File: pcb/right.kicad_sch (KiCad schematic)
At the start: 0 parts

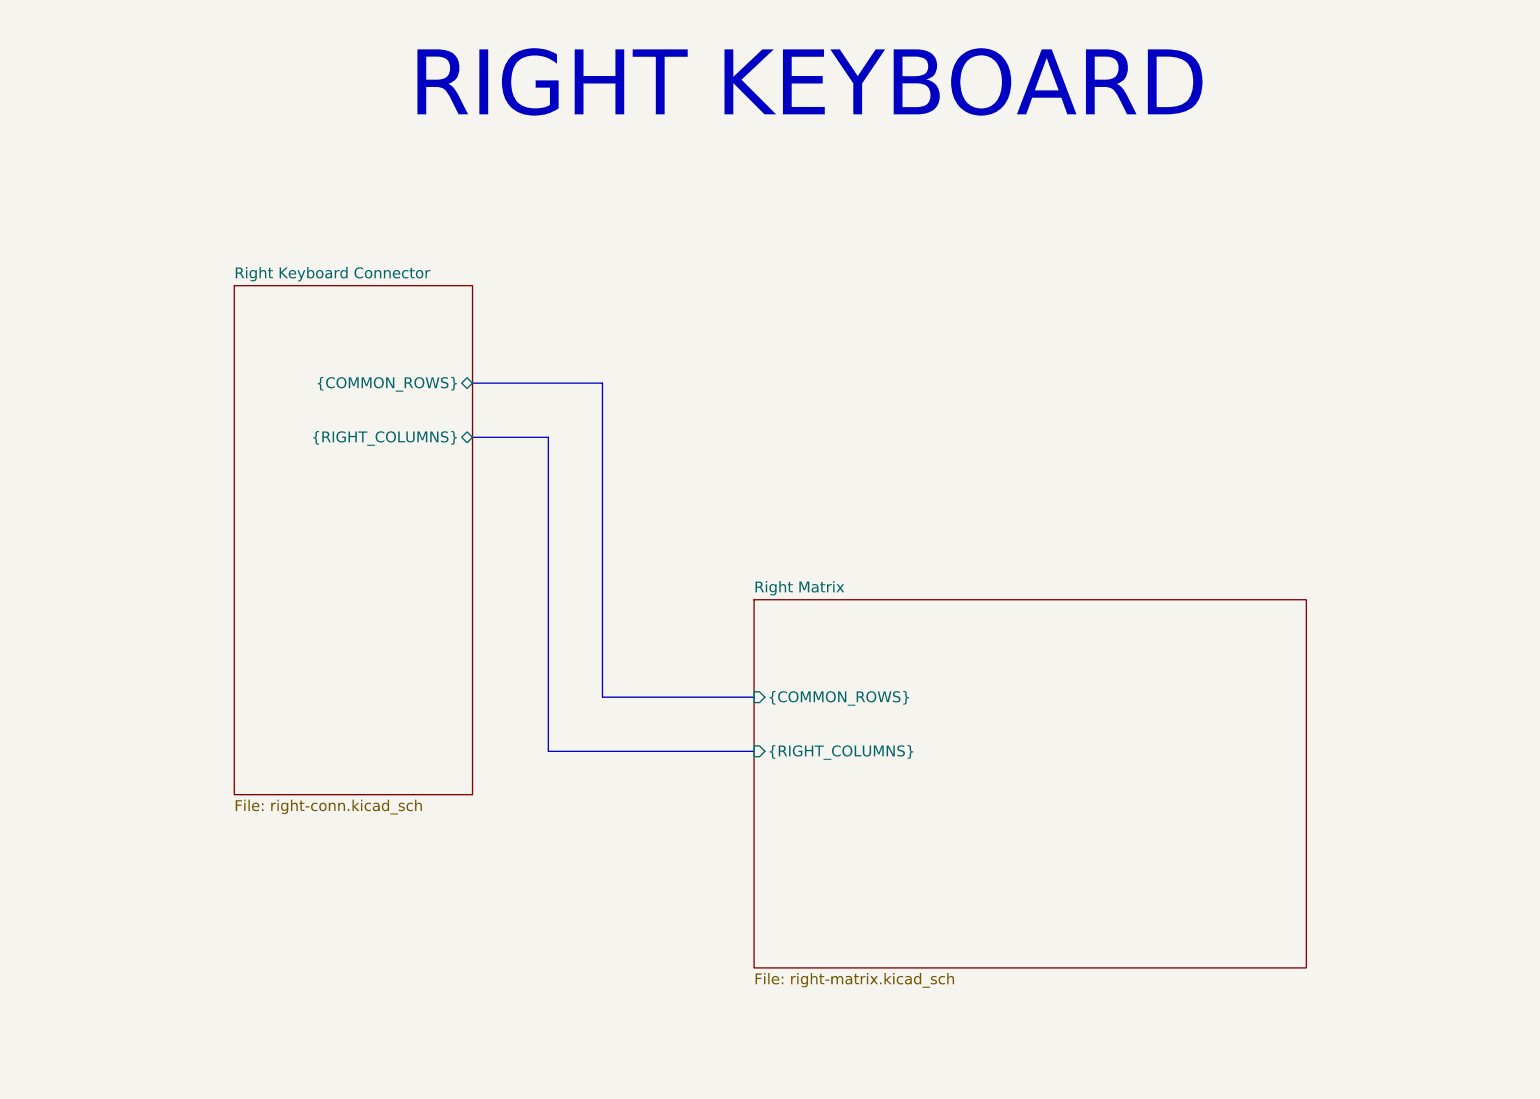
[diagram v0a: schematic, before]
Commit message: Figured out what GPIOs to use.
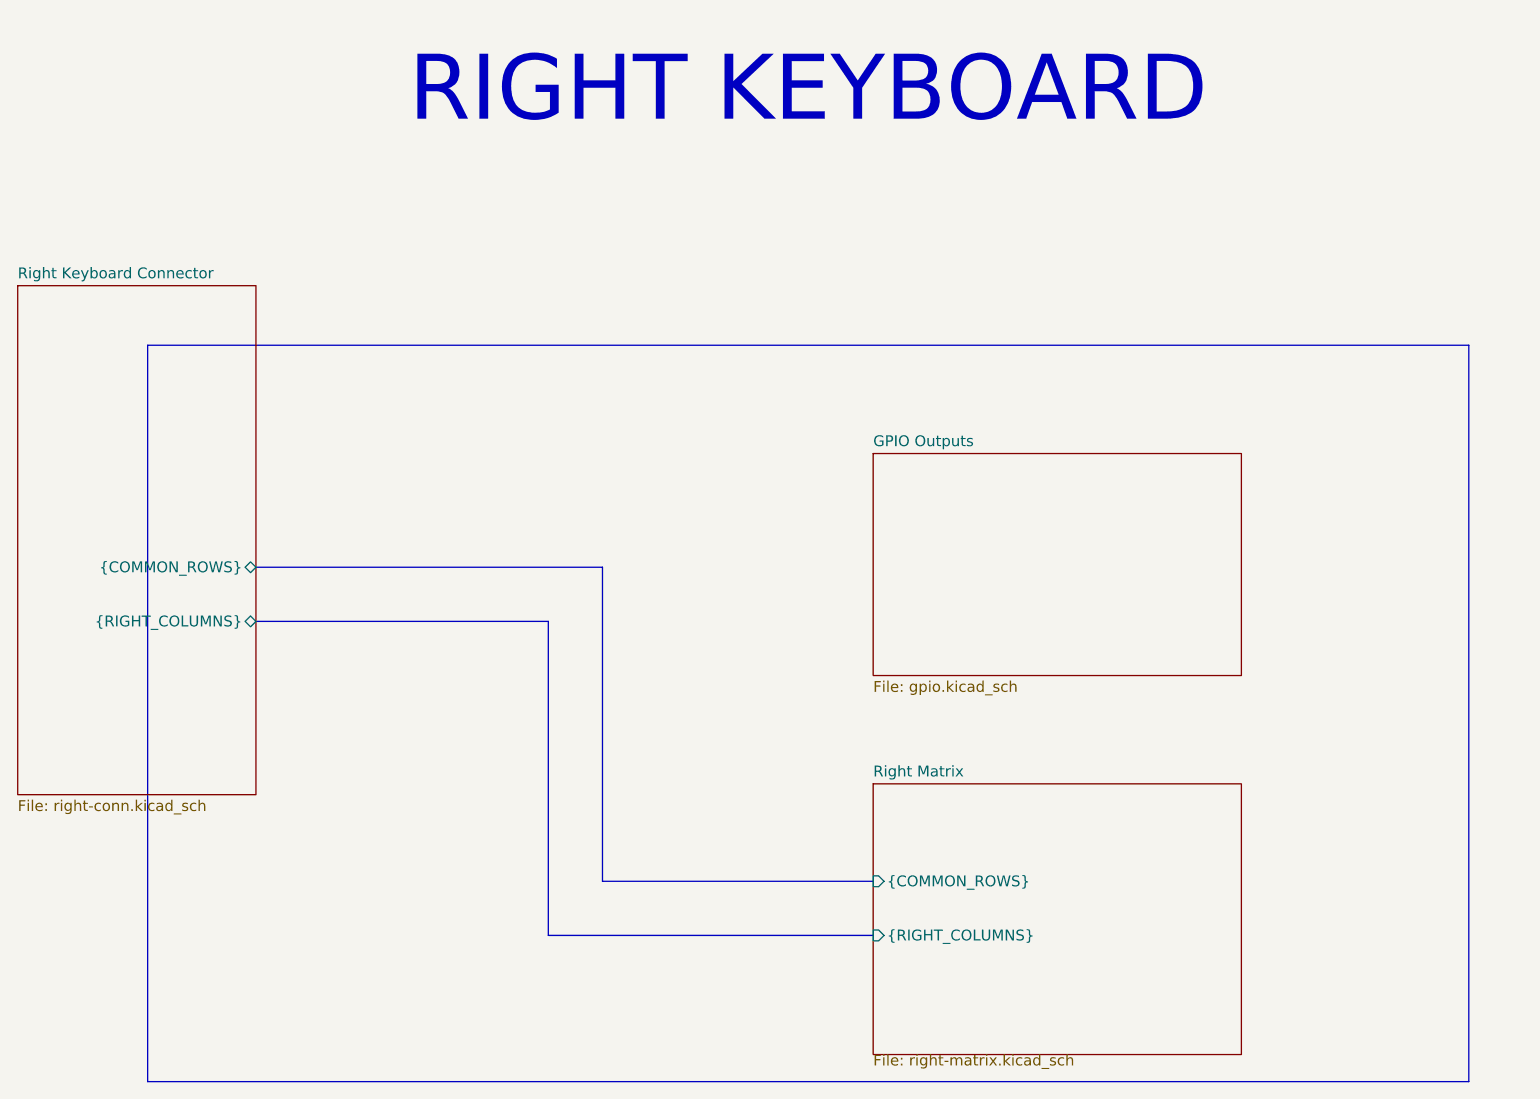
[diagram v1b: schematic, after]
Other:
- added sheet GPIO Outputs (gpio.kicad_sch)
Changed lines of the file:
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@@
 		(date "2025-06-11")
 	)
+	(rectangle
+		(start 73.66 62.865)
+		(end 228.6 149.225)
+		(stroke
+			(width 0)
+			(type solid)
+			(color 255 43 5 1)
+		)
+		(fill
+			(type none)
+		)
+	)
 	(text "RIGHT KEYBOARD"
 		(exclude_from_sim no)
-		(at 151.13 32.512 0)
+		(at 151.13 33.02 0)
 		(effects
 			(font
@@
 	(bus
 		(pts
-			(xy 127 67.31) (xy 111.76 67.31)
-		)
-		(stroke
-			(width 0)
-			(type default)
-		)
-	)
-	(bus
-		(pts
-			(xy 120.65 110.49) (xy 120.65 73.66)
-		)
-		(stroke
-			(width 0)
-			(type default)
-		)
-	)
-	(bus
-		(pts
-			(xy 120.65 110.49) (xy 144.78 110.49)
-		)
-		(stroke
-			(width 0)
-			(type default)
-		)
-	)
-	(bus
-		(pts
-			(xy 127 104.14) (xy 127 67.31)
-		)
-		(stroke
-			(width 0)
-			(type default)
-		)
-	)
-	(bus
-		(pts
-			(xy 120.65 73.66) (xy 111.76 73.66)
-		)
-		(stroke
-			(width 0)
-			(type default)
-		)
-	)
-	(bus
-		(pts
-			(xy 127 104.14) (xy 144.78 104.14)
+			(xy 127 88.9) (xy 86.36 88.9)
+		)
+		(stroke
+			(width 0)
+			(type default)
+		)
+	)
+	(bus
+		(pts
+			(xy 120.65 132.08) (xy 120.65 95.25)
+		)
+		(stroke
+			(width 0)
+			(type default)
+		)
+	)
+	(bus
+		(pts
+			(xy 120.65 132.08) (xy 158.75 132.08)
+		)
+		(stroke
+			(width 0)
+			(type default)
+		)
+	)
+	(bus
+		(pts
+			(xy 127 125.73) (xy 127 88.9)
+		)
+		(stroke
+			(width 0)
+			(type default)
+		)
+	)
+	(bus
+		(pts
+			(xy 120.65 95.25) (xy 86.36 95.25)
+		)
+		(stroke
+			(width 0)
+			(type default)
+		)
+	)
+	(bus
+		(pts
+			(xy 127 125.73) (xy 158.75 125.73)
 		)
 		(stroke
@@
 	)
 	(sheet
-		(at 83.82 55.88)
+		(at 58.42 55.88)
 		(size 27.94 59.69)
 		(exclude_from_sim no)
@@
 		)
 		(property "Sheetname" "Right Keyboard Connector"
-			(at 83.82 55.1684 0)
+			(at 58.42 55.1684 0)
 			(effects
 				(font
@@
 		)
 		(property "Sheetfile" "right-conn.kicad_sch"
-			(at 83.82 116.1546 0)
+			(at 58.42 116.1546 0)
 			(effects
 				(font
@@
 		)
 		(pin "{COMMON_ROWS}" bidirectional
-			(at 111.76 67.31 0)
+			(at 86.36 88.9 0)
 			(effects
 				(font
@@
 		)
 		(pin "{RIGHT_COLUMNS}" bidirectional
-			(at 111.76 73.66 0)
+			(at 86.36 95.25 0)
 			(effects
 				(font
@@
 	)
 	(sheet
-		(at 144.78 92.71)
-		(size 64.77 43.18)
+		(at 158.75 75.565)
+		(size 43.18 26.035)
 		(exclude_from_sim no)
 		(in_bom yes)
@@
 			(color 0 0 0 0.0000)
 		)
+		(property "Sheetname" "GPIO Outputs"
+			(at 158.75 74.8534 0)
+			(effects
+				(font
+					(size 1.27 1.27)
+				)
+				(justify left bottom)
+			)
+		)
+		(property "Sheetfile" "gpio.kicad_sch"
+			(at 158.75 102.1846 0)
+			(effects
+				(font
+					(size 1.27 1.27)
+				)
+				(justify left top)
+			)
+		)
+		(instances
+			(project "69split"
+				(path "/d75b0717-10e3-4e20-afcb-05300684210e/4b966fee-8f5c-4a23-a90e-d8e6cc86345c"
+					(page "10")
+				)
+			)
+		)
+	)
+	(sheet
+		(at 158.75 114.3)
+		(size 43.18 31.75)
+		(exclude_from_sim no)
+		(in_bom yes)
+		(on_board yes)
+		(dnp no)
+		(fields_autoplaced yes)
+		(stroke
+			(width 0.1524)
+			(type solid)
+		)
+		(fill
+			(color 0 0 0 0.0000)
+		)
 		(property "Sheetname" "Right Matrix"
-			(at 144.78 91.9984 0)
+			(at 158.75 113.5884 0)
 			(effects
 				(font
@@
 		)
 		(property "Sheetfile" "right-matrix.kicad_sch"
-			(at 144.78 136.4746 0)
+			(at 158.75 145.9996 0)
 			(effects
 				(font
@@
 		)
 		(pin "{COMMON_ROWS}" input
-			(at 144.78 104.14 180)
+			(at 158.75 125.73 180)
 			(effects
 				(font
@@
 		)
 		(pin "{RIGHT_COLUMNS}" input
-			(at 144.78 110.49 180)
-			(effects
-				(font
+			(at 158.75 132.08 180)
+			(effects
+				(font

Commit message: I think schematic is done?
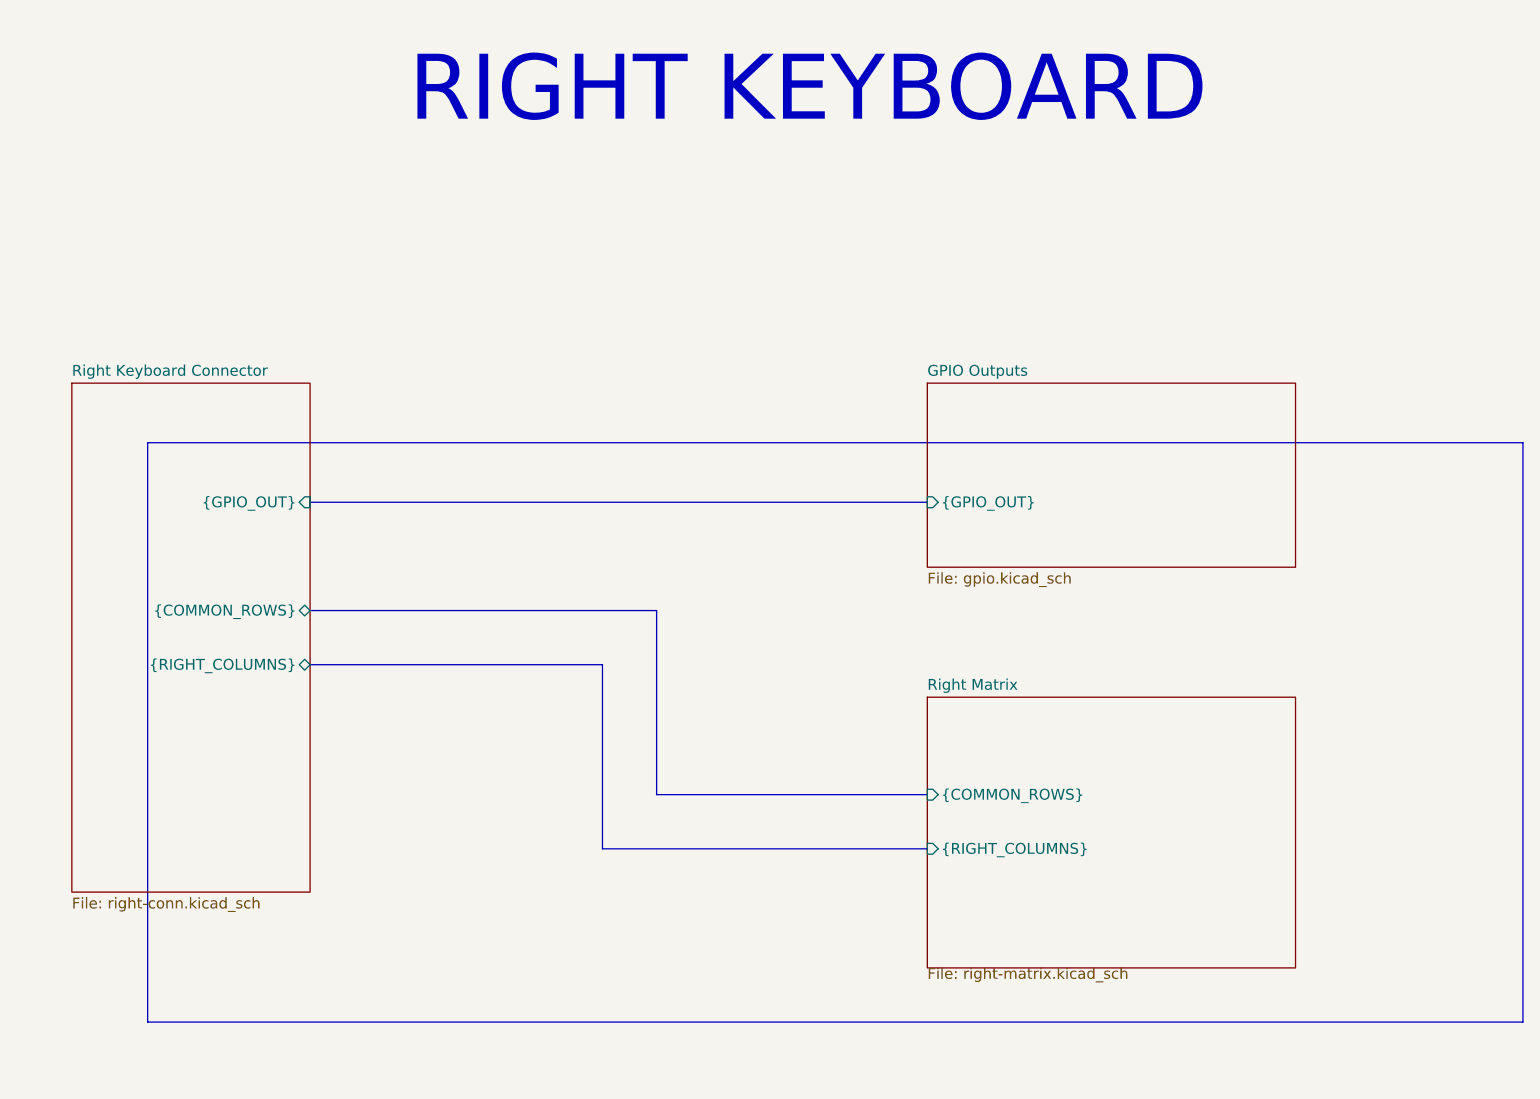
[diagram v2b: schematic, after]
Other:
- sheet GPIO Outputs ports: added {GPIO_OUT}; removed none
- sheet Right Keyboard Connector ports: added {GPIO_OUT}; removed none
- title: Split Normal 69 -> 69SPLIT KEYBOARD
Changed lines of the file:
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@@
 	(paper "A4")
 	(title_block
-		(title "Split Normal 69")
+		(title "69SPLIT KEYBOARD")
 		(date "2025-06-11")
 	)
 	(rectangle
-		(start 73.66 62.865)
-		(end 228.6 149.225)
+		(start 73.66 74.295)
+		(end 234.95 142.24)
 		(stroke
 			(width 0)
@@
 	(bus
 		(pts
-			(xy 127 88.9) (xy 86.36 88.9)
-		)
-		(stroke
-			(width 0)
-			(type default)
-		)
-	)
-	(bus
-		(pts
-			(xy 120.65 132.08) (xy 120.65 95.25)
-		)
-		(stroke
-			(width 0)
-			(type default)
-		)
-	)
-	(bus
-		(pts
-			(xy 120.65 132.08) (xy 158.75 132.08)
-		)
-		(stroke
-			(width 0)
-			(type default)
-		)
-	)
-	(bus
-		(pts
-			(xy 127 125.73) (xy 127 88.9)
-		)
-		(stroke
-			(width 0)
-			(type default)
-		)
-	)
-	(bus
-		(pts
-			(xy 120.65 95.25) (xy 86.36 95.25)
-		)
-		(stroke
-			(width 0)
-			(type default)
-		)
-	)
-	(bus
-		(pts
-			(xy 127 125.73) (xy 158.75 125.73)
+			(xy 133.35 93.98) (xy 92.71 93.98)
+		)
+		(stroke
+			(width 0)
+			(type default)
+		)
+	)
+	(bus
+		(pts
+			(xy 127 121.92) (xy 127 100.33)
+		)
+		(stroke
+			(width 0)
+			(type default)
+		)
+	)
+	(bus
+		(pts
+			(xy 127 121.92) (xy 165.1 121.92)
+		)
+		(stroke
+			(width 0)
+			(type default)
+		)
+	)
+	(bus
+		(pts
+			(xy 92.71 81.28) (xy 165.1 81.28)
+		)
+		(stroke
+			(width 0)
+			(type default)
+		)
+	)
+	(bus
+		(pts
+			(xy 133.35 115.57) (xy 133.35 93.98)
+		)
+		(stroke
+			(width 0)
+			(type default)
+		)
+	)
+	(bus
+		(pts
+			(xy 127 100.33) (xy 92.71 100.33)
+		)
+		(stroke
+			(width 0)
+			(type default)
+		)
+	)
+	(bus
+		(pts
+			(xy 133.35 115.57) (xy 165.1 115.57)
 		)
 		(stroke
@@
 	)
 	(sheet
-		(at 58.42 55.88)
+		(at 64.77 67.31)
 		(size 27.94 59.69)
 		(exclude_from_sim no)
@@
 		)
 		(property "Sheetname" "Right Keyboard Connector"
-			(at 58.42 55.1684 0)
+			(at 64.77 66.5984 0)
 			(effects
 				(font
@@
 		)
 		(property "Sheetfile" "right-conn.kicad_sch"
-			(at 58.42 116.1546 0)
+			(at 64.77 127.5846 0)
 			(effects
 				(font
@@
 		)
 		(pin "{COMMON_ROWS}" bidirectional
-			(at 86.36 88.9 0)
+			(at 92.71 93.98 0)
 			(effects
 				(font
@@
 		)
 		(pin "{RIGHT_COLUMNS}" bidirectional
-			(at 86.36 95.25 0)
+			(at 92.71 100.33 0)
 			(effects
 				(font
 					(size 1.27 1.27)
 					(thickness 0.1588)
+				)
+				(justify right)
+			)
+		)
+		(pin "{GPIO_OUT}" input
+			(at 92.71 81.28 0)
+			(effects
+				(font
+					(size 1.27 1.27)
 				)
 				(justify right)
@@
 	)
 	(sheet
-		(at 158.75 75.565)
-		(size 43.18 26.035)
+		(at 165.1 67.31)
+		(size 43.18 21.59)
 		(exclude_from_sim no)
 		(in_bom yes)
@@
 		)
 		(property "Sheetname" "GPIO Outputs"
-			(at 158.75 74.8534 0)
+			(at 165.1 66.5984 0)
 			(effects
 				(font
@@
 		)
 		(property "Sheetfile" "gpio.kicad_sch"
-			(at 158.75 102.1846 0)
+			(at 165.1 89.4846 0)
 			(effects
 				(font
@@
 				)
 				(justify left top)
+			)
+		)
+		(pin "{GPIO_OUT}" input
+			(at 165.1 81.28 180)
+			(effects
+				(font
+					(size 1.27 1.27)
+				)
+				(justify left)
 			)
 		)
@@
 	)
 	(sheet
-		(at 158.75 114.3)
+		(at 165.1 104.14)
 		(size 43.18 31.75)
 		(exclude_from_sim no)
@@
 		)
 		(property "Sheetname" "Right Matrix"
-			(at 158.75 113.5884 0)
+			(at 165.1 103.4284 0)
 			(effects
 				(font
@@
 		)
 		(property "Sheetfile" "right-matrix.kicad_sch"
-			(at 158.75 145.9996 0)
+			(at 165.1 135.8396 0)
 			(effects
 				(font
@@
 		)
 		(pin "{COMMON_ROWS}" input
-			(at 158.75 125.73 180)
+			(at 165.1 115.57 180)
 			(effects
 				(font
@@
 		)
 		(pin "{RIGHT_COLUMNS}" input
-			(at 158.75 132.08 180)
-			(effects
-				(font
+			(at 165.1 121.92 180)
+			(effects
+				(font
